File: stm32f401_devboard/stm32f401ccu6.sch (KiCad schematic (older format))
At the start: 29 parts, among them CON1 CORTEX-DEBUGGER, J1 microusb, SW1 SW_Push, SW2 SW_Push, SW3 SW_Push, U1 STM32F401CCUx, U2 LM1117-3.3, Y1 12MHz, Y2 32.768K

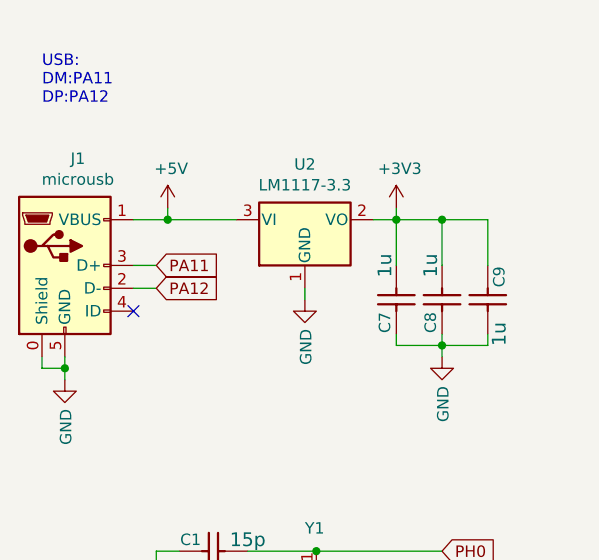
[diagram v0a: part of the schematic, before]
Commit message: usb fix
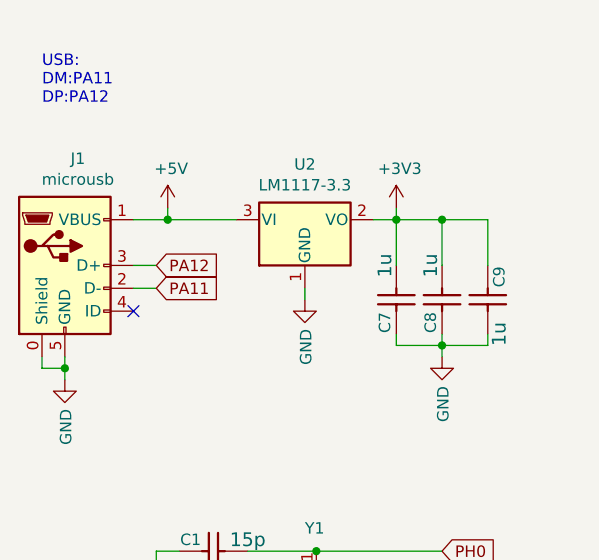
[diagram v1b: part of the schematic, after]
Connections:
- net PA11: now also J1.2 (D-); no longer J1.3 (D+)
- net PA12: now also J1.3 (D+); no longer J1.2 (D-)
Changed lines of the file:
@@
 	1450 1650 1350 1650
 Text GLabel 1450 1550 2    50   Input ~ 0
+PA12
+Text GLabel 1450 1650 2    50   Input ~ 0
 PA11
-Text GLabel 1450 1650 2    50   Input ~ 0
-PA12
 $Comp
 L Regulator_Linear:LM1117-3.3 U2
